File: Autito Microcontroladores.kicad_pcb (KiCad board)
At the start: 2 copper layers, 81.2 x 115.3 mm, 87 parts, among them J1 SENSOR 1, J10 USB, J11 SWD, J12 BOOT MODE, J13 Batería2, J14 Bateria1, J2 SENSOR 4, J3 SENSOR 2, J4 SENSOR 5, J5 SENSOR 3, J6 SENSOR 6, J7 Motor izquierda, J8 Motor derecha, J9 Flash enable, SW1 RESET, SW2 PID Init, SW3 RESET, U1 L9110, U2 L9110, U3 ESP-12F, U4 STM32F103C8Tx, U5 LM2596S-5, U6 AMS1117-3.3, Y1 8MHz

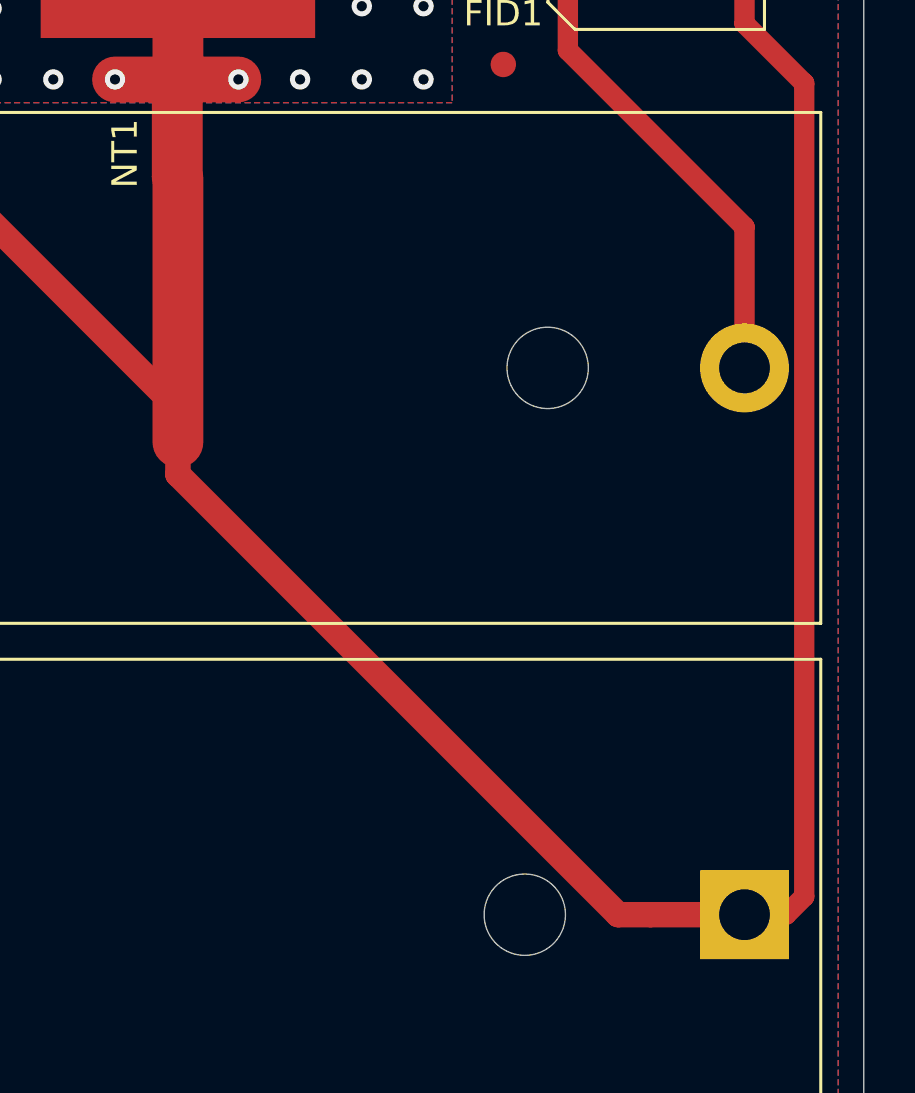
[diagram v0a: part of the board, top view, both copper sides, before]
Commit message: Entrega
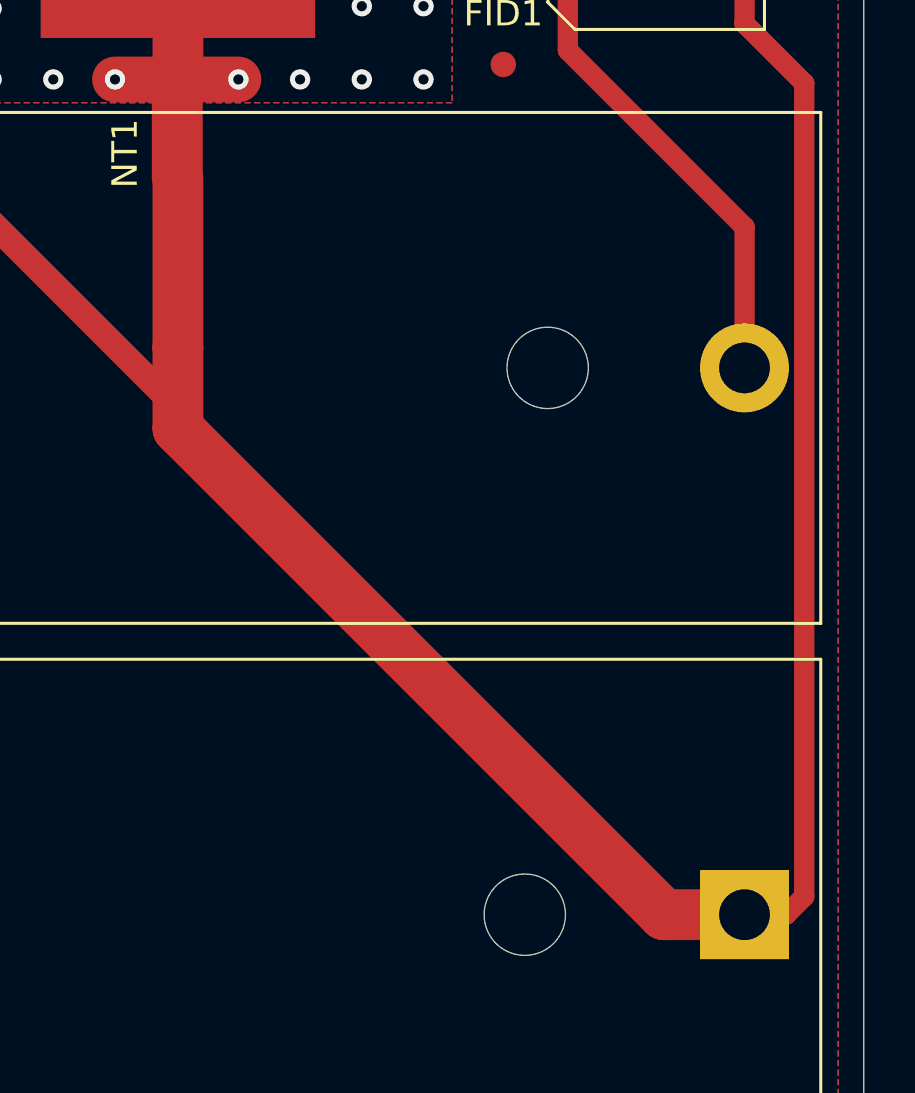
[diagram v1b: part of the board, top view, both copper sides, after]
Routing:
- net GNDREF: track 513.9 -> 512.9 mm
